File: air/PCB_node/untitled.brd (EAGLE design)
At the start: 109 x 66 mm, 31 parts, among them K1 351, K2 351, Q1 S9013, Q2 S9013, U1 ESP32-DEVKITC-32D, U2 PC817X2NIP0F, U3 PC817X2NIP0F, X1 MSTBA2, X2 MSTBA5, X3 MSTBA2, X4 MSTBA2, X5 MSTBA2

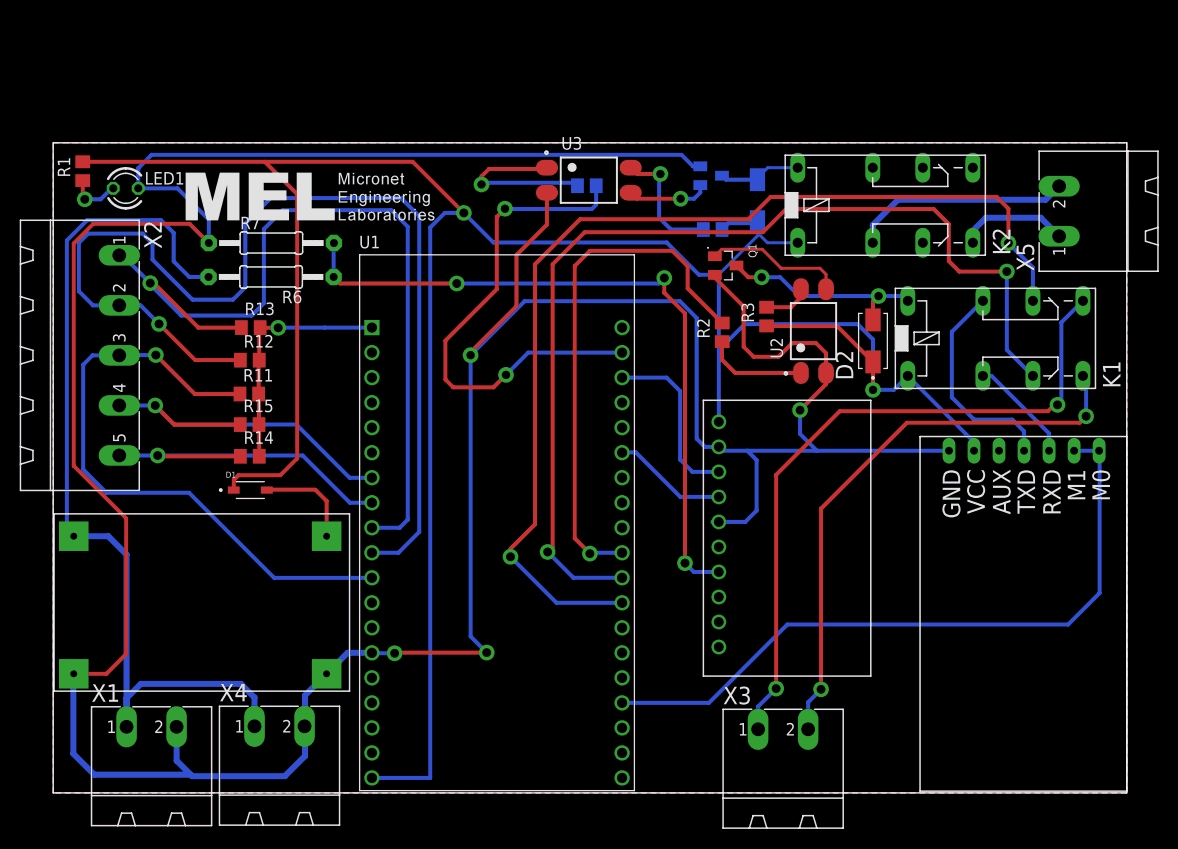
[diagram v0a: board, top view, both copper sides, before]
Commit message: revisi tanggal 24/02/2023
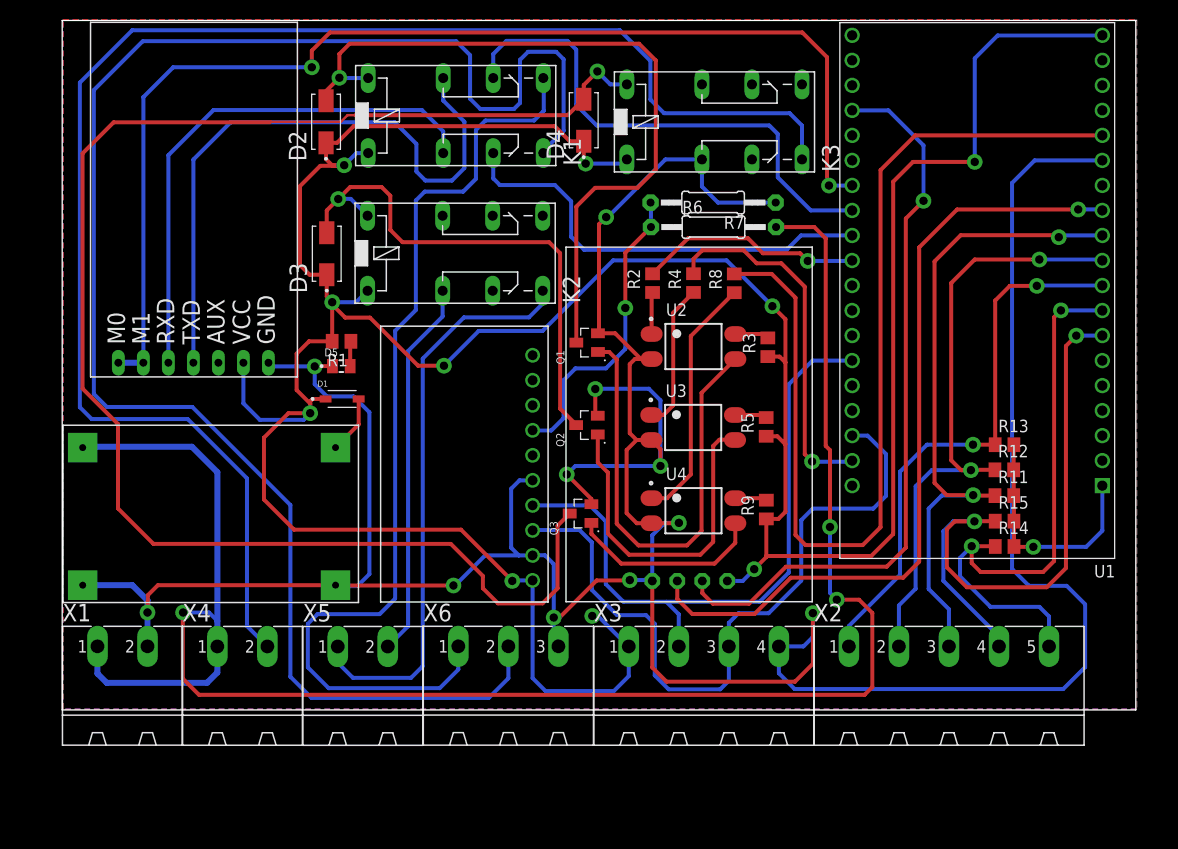
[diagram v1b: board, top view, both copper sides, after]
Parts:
- removed LED1: TLLY4400, led:LED3MM
- added D4: US1M-13, US1M-13:DIOM5226X240N
- added D5: SML-LXT0805IW-TR, SML-LXT0805IW-TR:LEDC2012X120N
- added K3: 351, relay:351
- added NEO-6MGPS1: (no value), NEO-6M GPS:NEO-6MGPS
- added Q3: S9013, S9013:SOT95P240X120-3N
- added R8, R9: (no value), rcl:R0805
- added U4: PC817X2NIP0F, PC817X2NIP0F:SOT254P975X400-4N
- added X6: MSTBA3, con-phoenix-508:MSTBA3
- X3: value MSTBA2 -> MSTBA4; device con-phoenix-508:MSTBA2 -> con-phoenix-508:MSTBA4
- moved EBYTEE220-900T22D1 102.8 mm to (5.79, 48.2), turned to 90 degrees
- moved X2 95.8 mm to (90.9, 9.79), turned to 0 degrees
- moved X5 90.4 mm to (31.4, 9.78), turned to 0 degrees
- moved R13 77.4 mm to (96.6, 35.3)
- moved R12 77.4 mm to (96.6, 32.8)
- moved R11 77.3 mm to (96.6, 30.2)
- moved R15 77.3 mm to (96.6, 27.6)
- moved R14 77.2 mm to (96.6, 25.0)
- moved D2 59.8 mm to (27.7, 68.1)
- moved K1 59.3 mm to (35.8, 68.8)
- moved U1 54.1 mm to (93.8, 51.0), turned to 180 degrees
- moved R6 45.2 mm to (67.0, 57.4), turned to 0 degrees
- moved R7 45.0 mm to (67.0, 59.9), turned to 180 degrees
- moved D3 44.1 mm to (27.8, 54.7), flipped to the top
- moved K2 43.9 mm to (35.7, 54.8)
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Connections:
- new net GND-VALVE: K3.S1, X4.2
- new net N$11: Q3.1, U4.3
- new net N$13: D4.A, K3.16, Q3.3
- new net N$4: R8.1, U4.1
- new net N$8: R9.2, U4.4
- new net RX_GPS: NEO-6MGPS1.RX, U1.35
- new net TX_GPS: NEO-6MGPS1.TX, U1.12
- new net VALVE-POWER: R8.2, U1.15
- net GND: now also D5.C, K3.P1, NEO-6MGPS1.GND, Q3.2, U4.2, X3.4, X6.3; no longer LED1.K, X4.2
- net M0: now also U1.32; no longer U1.35
- net N$1: now also D5.A; no longer LED1.A
- net RXLORA_CONFIG: now also X6.2; no longer X3.2
- net SCL: now also X3.3
- net SDA: now also X3.2
- net TXLORA_CONFIG: now also X6.1; no longer X3.1
- net VCC: now also D4.C, K3.1, NEO-6MGPS1.5V, R9.1, X3.1
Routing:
- net GND-VALVE: track 0.00 -> 156.1 mm
- net N$13: track 0.00 -> 155.7 mm, vias 0 -> 1
- net RXLORA_CONFIG: track 58.0 -> 170.9 mm, vias 2 -> 0
- net VALVE-POWER: track 0.00 -> 101.4 mm
- net 24V: track 93.3 -> 186.8 mm, vias 0 -> 3
- net VCC: track 257.5 -> 339.1 mm, vias 2 -> 10
- net TX_GPS: track 0.00 -> 81.4 mm, vias 0 -> 1
- net RX_GPS: track 0.00 -> 75.0 mm, vias 0 -> 1
- net RXLORA_MICRO: track 103.0 -> 44.7 mm, vias 2 -> 0
- net SDA: track 11.7 -> 66.6 mm
- net SCL: track 17.9 -> 72.1 mm
- net TXLORA_MICRO: track 105.9 -> 52.4 mm, vias 2 -> 0
- net N$6: track 22.7 -> 76.0 mm, vias 2 -> 1
- net M0: track 70.3 -> 119.1 mm, vias 0 -> 2
- net VALVE1: track 11.3 -> 58.4 mm
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- added copper zone on layer 1, net N$15
- added copper zone on layer 16, net N$16
- removed copper zone on layer 1, net N$4
- removed copper zone on layer 16, net N$8
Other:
- board size 109 x 66 mm -> 109 x 70 mm
